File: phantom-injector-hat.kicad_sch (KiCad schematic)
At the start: 41 parts, among them J1 Conn_02x20_Odd_Even, J2 Conn_02x03_Top_Bottom, J3 Conn_01x03, J4 Conn_01x03, SW1 SW_SPST, SW2 SW_SPST, U1 LT8362EMSE-PBF

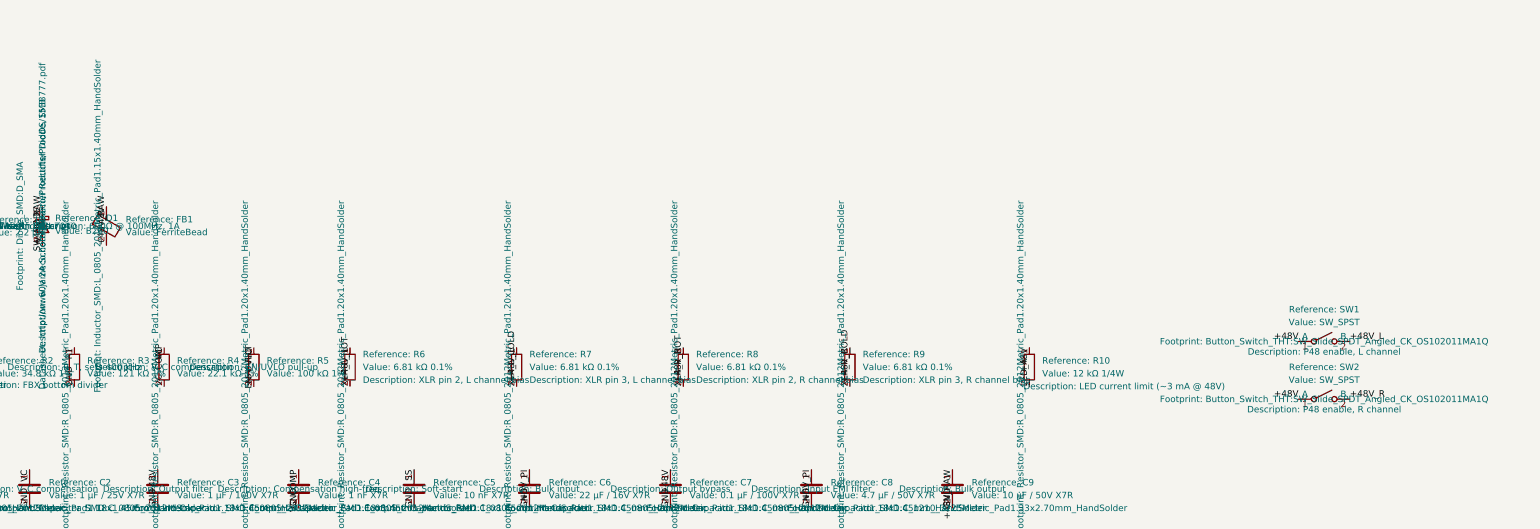
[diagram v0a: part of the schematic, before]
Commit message: checkpoint before final layout and wiring
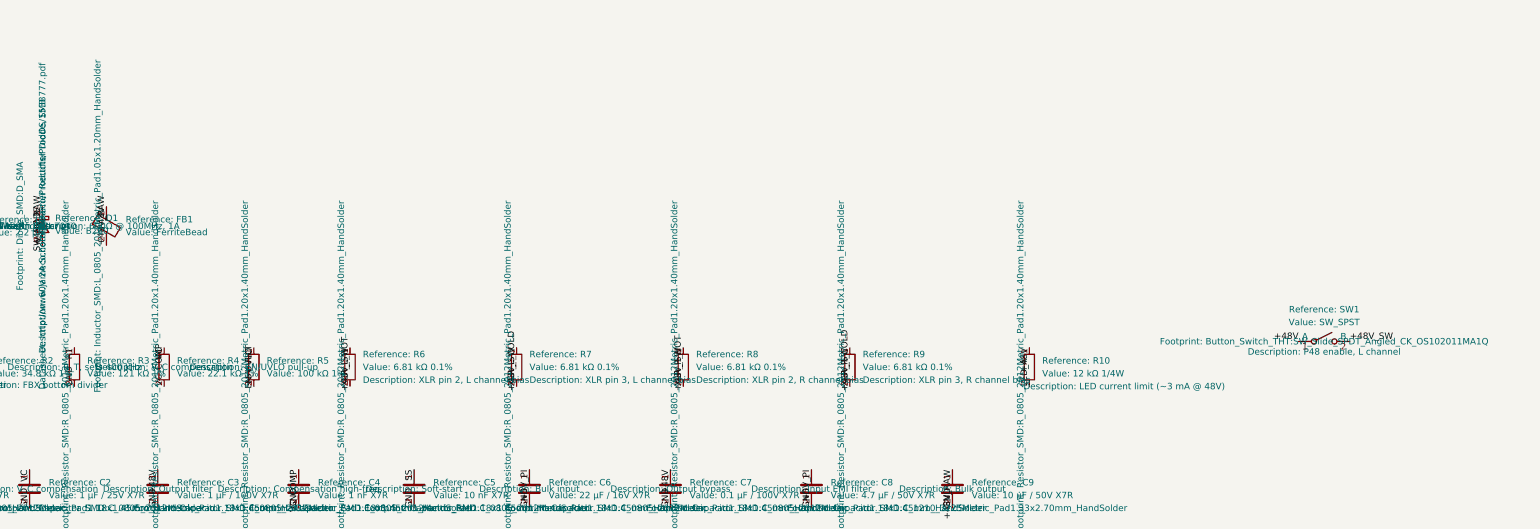
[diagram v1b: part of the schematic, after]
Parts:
- removed SW2: SW_SPST, Button_Switch_THT:SW_Slide_SPDT_Angled_CK_OS102011MA1Q, symbol Switch:SW_SPST
- FB1: footprint Inductor_SMD:L_0805_2012Metric_Pad1.15x1.40mm_HandSolder -> Inductor_SMD:L_0805_2012Metric_Pad1.05x1.20mm_HandSolder
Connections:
- net +48V_R is gone; now on net +48V_SW: R8.1, R9.1
- net +48V_L renamed +48V_SW

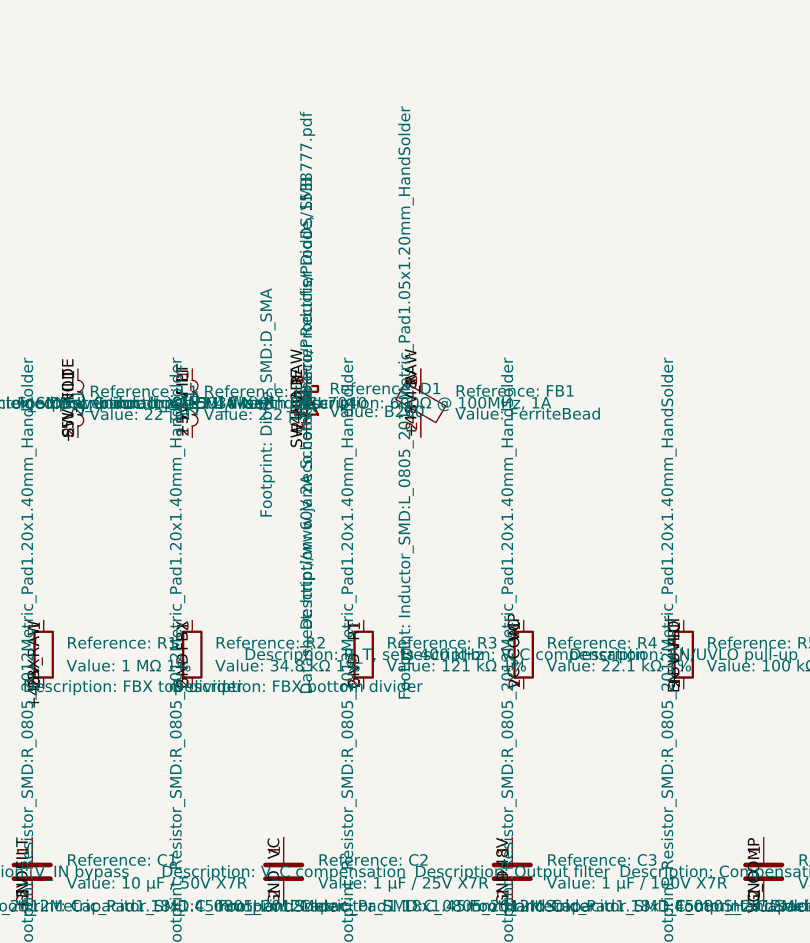
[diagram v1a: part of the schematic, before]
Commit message: CHeckpoint
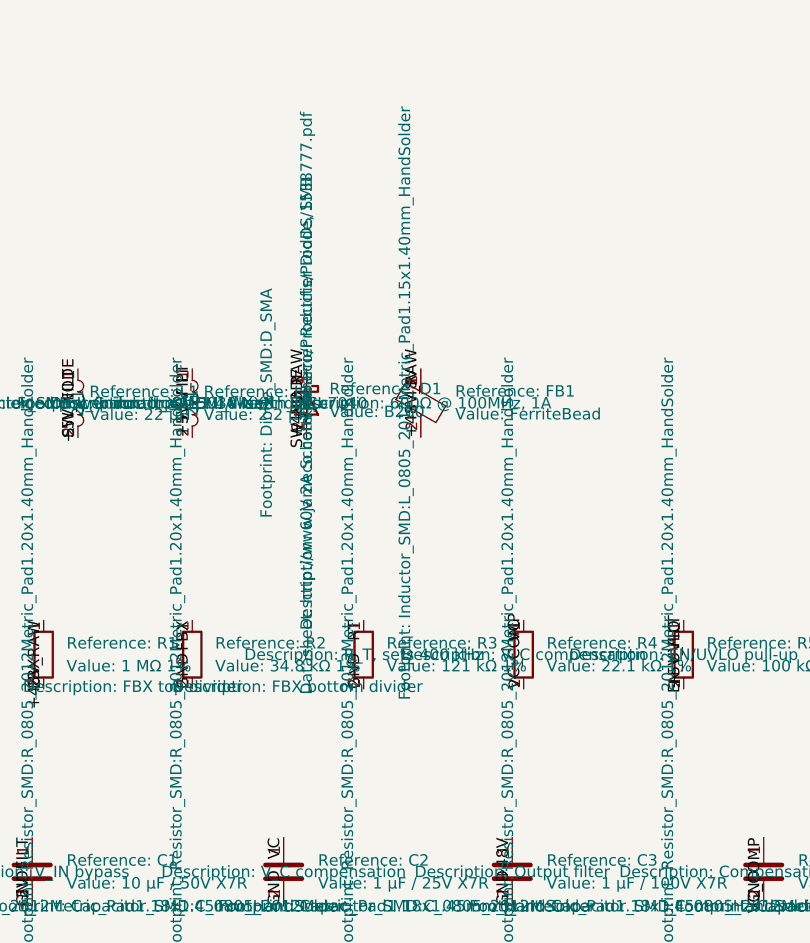
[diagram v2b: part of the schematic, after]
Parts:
- FB1: footprint Inductor_SMD:L_0805_2012Metric_Pad1.05x1.20mm_HandSolder -> Inductor_SMD:L_0805_2012Metric_Pad1.15x1.40mm_HandSolder
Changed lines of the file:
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@@
 			)
 		)
-		(property "Footprint" "Inductor_SMD:L_0805_2012Metric_Pad1.05x1.20mm_HandSolder"
+		(property "Footprint" "Inductor_SMD:L_0805_2012Metric_Pad1.15x1.40mm_HandSolder"
 			(at 76.962 30.48 90)
 			(show_name yes)

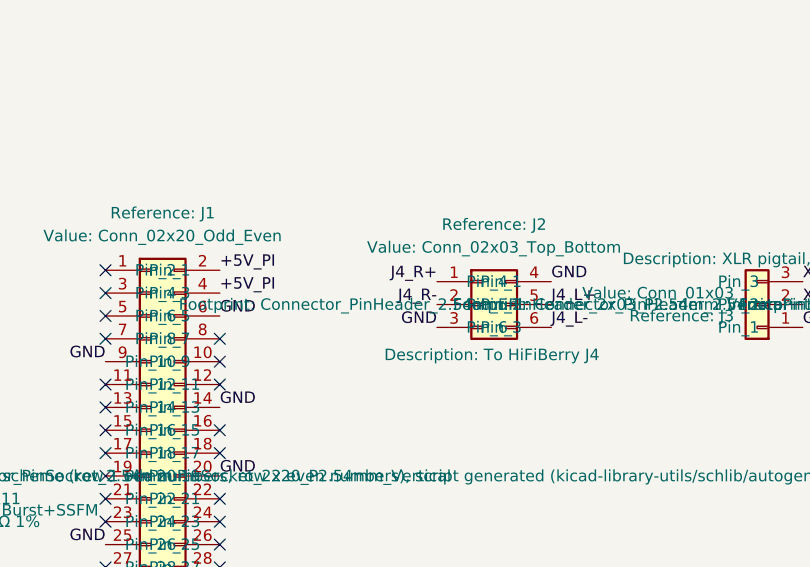
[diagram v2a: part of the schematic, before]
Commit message: Checkpoint!
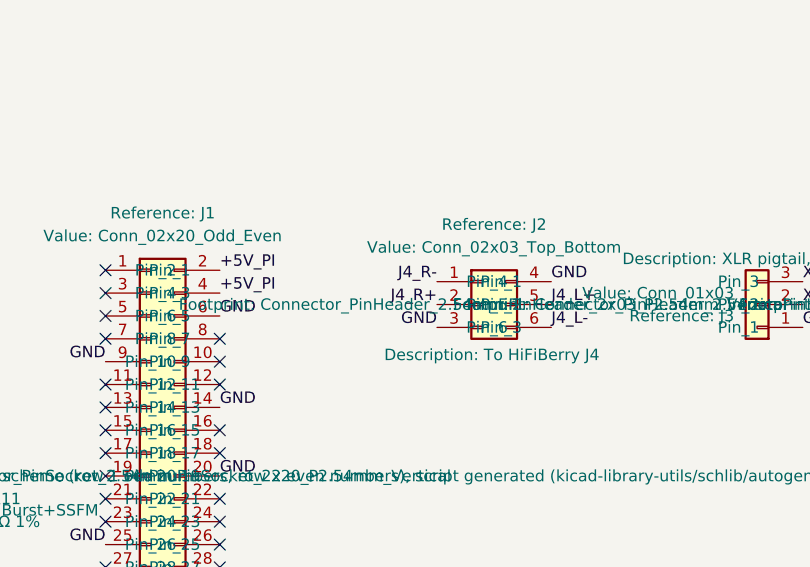
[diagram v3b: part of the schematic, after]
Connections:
- net J4_R+: now also J2.2 (Pin_2); no longer J2.1 (Pin_1)
- net J4_R-: now also J2.1 (Pin_1); no longer J2.2 (Pin_2)
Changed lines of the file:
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@@
 	)
 	(label "J4_R-"
-		(at 176.53 162.56 180)
+		(at 176.53 160.02 180)
 		(effects
 			(font
@@
 	)
 	(label "J4_R+"
-		(at 176.53 160.02 180)
-		(effects
-			(font
+		(at 176.53 162.56 180)
+		(effects
+			(font

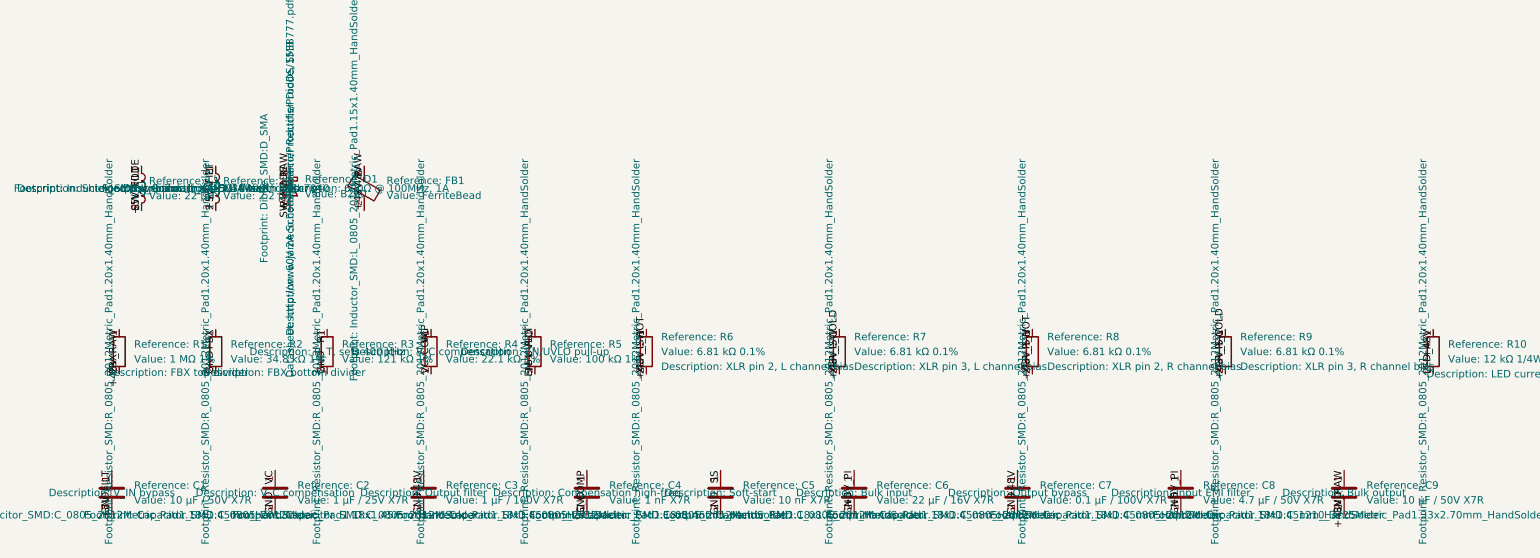
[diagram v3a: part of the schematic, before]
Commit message: Checkpoint
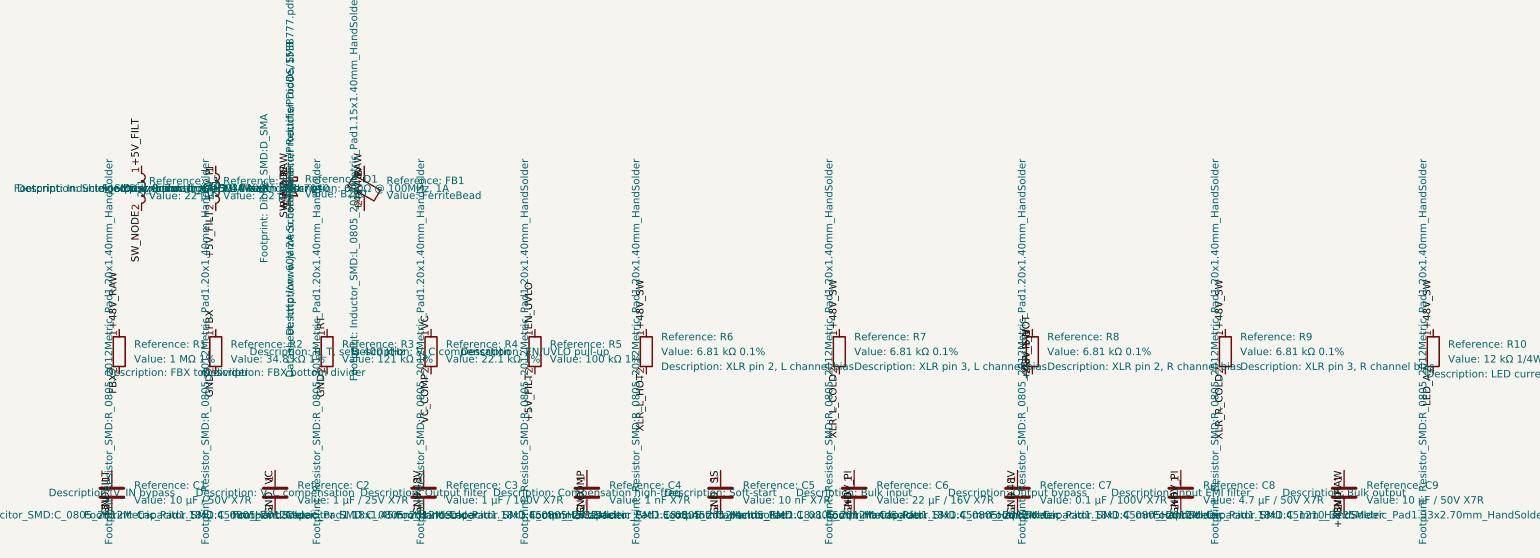
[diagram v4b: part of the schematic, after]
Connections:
- net +48V: no longer R10.1
- net +48V_SW: now also R10.1
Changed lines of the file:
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@@
 	)
 	(label "FBX"
-		(at 36.83 62.23 90)
-		(effects
-			(font
-				(size 1.27 1.27)
-			)
-			(justify left bottom)
+		(at 36.83 62.23 270)
+		(effects
+			(font
+				(size 1.27 1.27)
+			)
+			(justify right bottom)
 		)
 	)
@@
 	)
 	(label "XLR_L_HOT"
-		(at 127 62.23 90)
-		(effects
-			(font
-				(size 1.27 1.27)
-			)
-			(justify left bottom)
+		(at 127 62.23 270)
+		(effects
+			(font
+				(size 1.27 1.27)
+			)
+			(justify right bottom)
 		)
 	)
@@
 	)
 	(label "XLR_R_COLD"
-		(at 226.06 62.23 90)
-		(effects
-			(font
-				(size 1.27 1.27)
-			)
-			(justify left bottom)
+		(at 226.06 62.23 270)
+		(effects
+			(font
+				(size 1.27 1.27)
+			)
+			(justify right bottom)
 		)
 	)
@@
 	)
 	(label "GND"
-		(at 72.39 62.23 90)
-		(effects
-			(font
-				(size 1.27 1.27)
-			)
-			(justify left bottom)
+		(at 72.39 62.23 270)
+		(effects
+			(font
+				(size 1.27 1.27)
+			)
+			(justify right bottom)
 		)
 	)
 	(label "+48V_SW"
-		(at 160.02 54.61 270)
-		(effects
-			(font
-				(size 1.27 1.27)
-			)
-			(justify right bottom)
+		(at 160.02 54.61 90)
+		(effects
+			(font
+				(size 1.27 1.27)
+			)
+			(justify left bottom)
 		)
 	)
@@
 	)
 	(label "+48V_RAW"
-		(at 36.83 54.61 270)
-		(effects
-			(font
-				(size 1.27 1.27)
-			)
-			(justify right bottom)
+		(at 36.83 54.61 90)
+		(effects
+			(font
+				(size 1.27 1.27)
+			)
+			(justify left bottom)
 		)
 	)
@@
 	)
 	(label "XLR_L_COLD"
-		(at 160.02 62.23 90)
-		(effects
-			(font
-				(size 1.27 1.27)
-			)
-			(justify left bottom)
-		)
-	)
-	(label "GND"
-		(at 53.34 62.23 90)
-		(effects
-			(font
-				(size 1.27 1.27)
-			)
-			(justify left bottom)
+		(at 160.02 62.23 270)
+		(effects
+			(font
+				(size 1.27 1.27)
+			)
+			(justify right bottom)
+		)
+	)
+	(label "GND"
+		(at 53.34 62.23 270)
+		(effects
+			(font
+				(size 1.27 1.27)
+			)
+			(justify right bottom)
 		)
 	)
 	(label "SW_NODE"
-		(at 40.64 34.29 90)
-		(effects
-			(font
-				(size 1.27 1.27)
-			)
-			(justify left bottom)
+		(at 40.64 34.29 270)
+		(effects
+			(font
+				(size 1.27 1.27)
+			)
+			(justify right bottom)
 		)
 	)
@@
 	)
 	(label "+5V_FILT"
-		(at 53.34 34.29 90)
-		(effects
-			(font
-				(size 1.27 1.27)
-			)
-			(justify left bottom)
+		(at 53.34 34.29 270)
+		(effects
+			(font
+				(size 1.27 1.27)
+			)
+			(justify right bottom)
 		)
 	)
@@
 	)
 	(label "+5V_FILT"
-		(at 107.95 62.23 90)
-		(effects
-			(font
-				(size 1.27 1.27)
-			)
-			(justify left bottom)
+		(at 107.95 62.23 270)
+		(effects
+			(font
+				(size 1.27 1.27)
+			)
+			(justify right bottom)
 		)
 	)
 	(label "+48V_SW"
-		(at 127 54.61 270)
-		(effects
-			(font
-				(size 1.27 1.27)
-			)
-			(justify right bottom)
+		(at 127 54.61 90)
+		(effects
+			(font
+				(size 1.27 1.27)
+			)
+			(justify left bottom)
 		)
 	)
@@
 	)
 	(label "EN_UVLO"
-		(at 107.95 54.61 270)
-		(effects
-			(font
-				(size 1.27 1.27)
-			)
-			(justify right bottom)
+		(at 107.95 54.61 90)
+		(effects
+			(font
+				(size 1.27 1.27)
+			)
+			(justify left bottom)
 		)
 	)
 	(label "VC_COMP"
-		(at 90.17 62.23 90)
-		(effects
-			(font
-				(size 1.27 1.27)
-			)
-			(justify left bottom)
+		(at 90.17 62.23 270)
+		(effects
+			(font
+				(size 1.27 1.27)
+			)
+			(justify right bottom)
 		)
 	)
@@
 	)
 	(label "LED_A"
-		(at 261.62 62.23 90)
-		(effects
-			(font
-				(size 1.27 1.27)
-			)
-			(justify left bottom)
+		(at 261.62 62.23 270)
+		(effects
+			(font
+				(size 1.27 1.27)
+			)
+			(justify right bottom)
 		)
 	)
@@
 		)
 	)
-	(label "+48V"
-		(at 261.62 54.61 270)
-		(effects
-			(font
-				(size 1.27 1.27)
-			)
-			(justify right bottom)
-		)
-	)
 	(label "+48V_SW"
-		(at 226.06 54.61 270)
-		(effects
-			(font
-				(size 1.27 1.27)
-			)
-			(justify right bottom)
+		(at 226.06 54.61 90)
+		(effects
+			(font
+				(size 1.27 1.27)
+			)
+			(justify left bottom)
 		)
 	)
@@
 	)
 	(label "+5V_FILT"
-		(at 40.64 26.67 270)
-		(effects
-			(font
-				(size 1.27 1.27)
-			)
-			(justify right bottom)
+		(at 40.64 26.67 90)
+		(effects
+			(font
+				(size 1.27 1.27)
+			)
+			(justify left bottom)
 		)
 	)
@@
 	)
 	(label "FBX"
-		(at 53.34 54.61 270)
-		(effects
-			(font
-				(size 1.27 1.27)
-			)
-			(justify right bottom)
+		(at 53.34 54.61 90)
+		(effects
+			(font
+				(size 1.27 1.27)
+			)
+			(justify left bottom)
 		)
 	)
@@
 	)
 	(label "RT"
-		(at 72.39 54.61 270)
-		(effects
-			(font
-				(size 1.27 1.27)
-			)
-			(justify right bottom)
+		(at 72.39 54.61 90)
+		(effects
+			(font
+				(size 1.27 1.27)
+			)
+			(justify left bottom)
+		)
+	)
+	(label "+48V_SW"
+		(at 261.62 54.61 90)
+		(effects
+			(font
+				(size 1.27 1.27)
+			)
+			(justify left bottom)
 		)
 	)
@@
 	)
 	(label "VC"
-		(at 90.17 54.61 270)
-		(effects
-			(font
-				(size 1.27 1.27)
-			)
-			(justify right bottom)
-		)
-	)
+		(at 90.17 54.61 90)
+		(effects
+			(font
+				(size 1.27 1.27)
+			)
+			(justify left bottom)
+		)
+	)
